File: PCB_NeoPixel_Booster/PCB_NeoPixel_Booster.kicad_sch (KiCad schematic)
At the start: 22 parts, among them J1 Power_Input_Screw, J10 Power_Breakout, J11 Power_Input_Screw, J12 REG_CONTROL, J2 Power_Input_Barrel_Jack, J3 Vcc_Breakout, J4 LED_Strip_Connector, J5 Power_Input_Screw, J6 LED_Strip_Connector, J7 Data_Input, J8 Power_Breakout, U1 AP2210K-5.0, U3 74LVC2G34GW

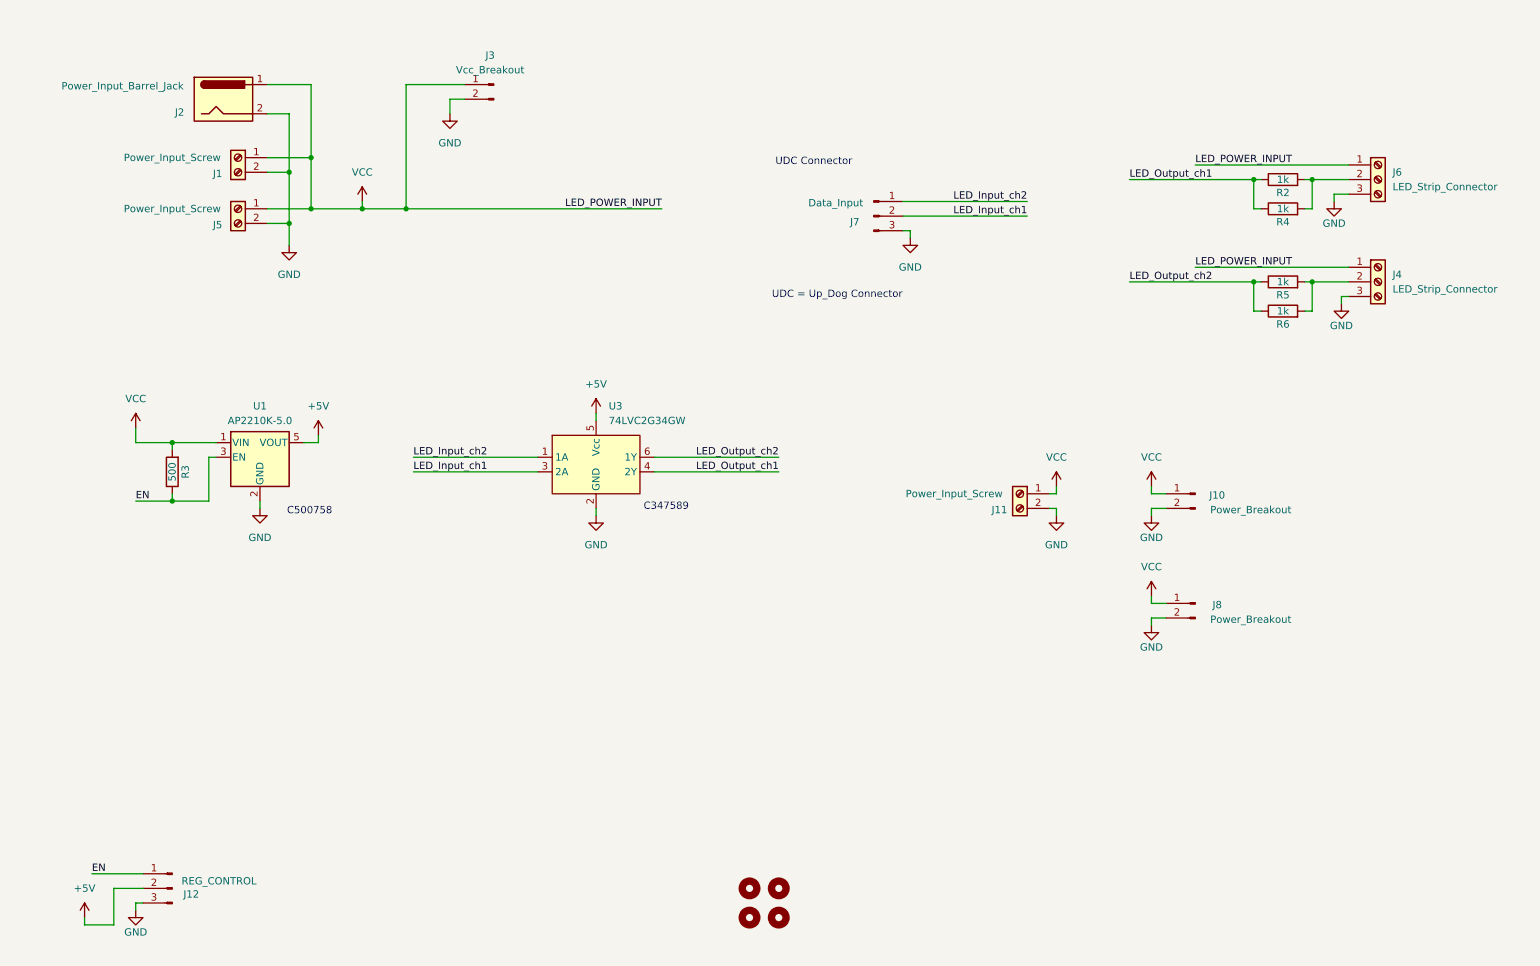
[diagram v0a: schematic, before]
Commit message: Fin
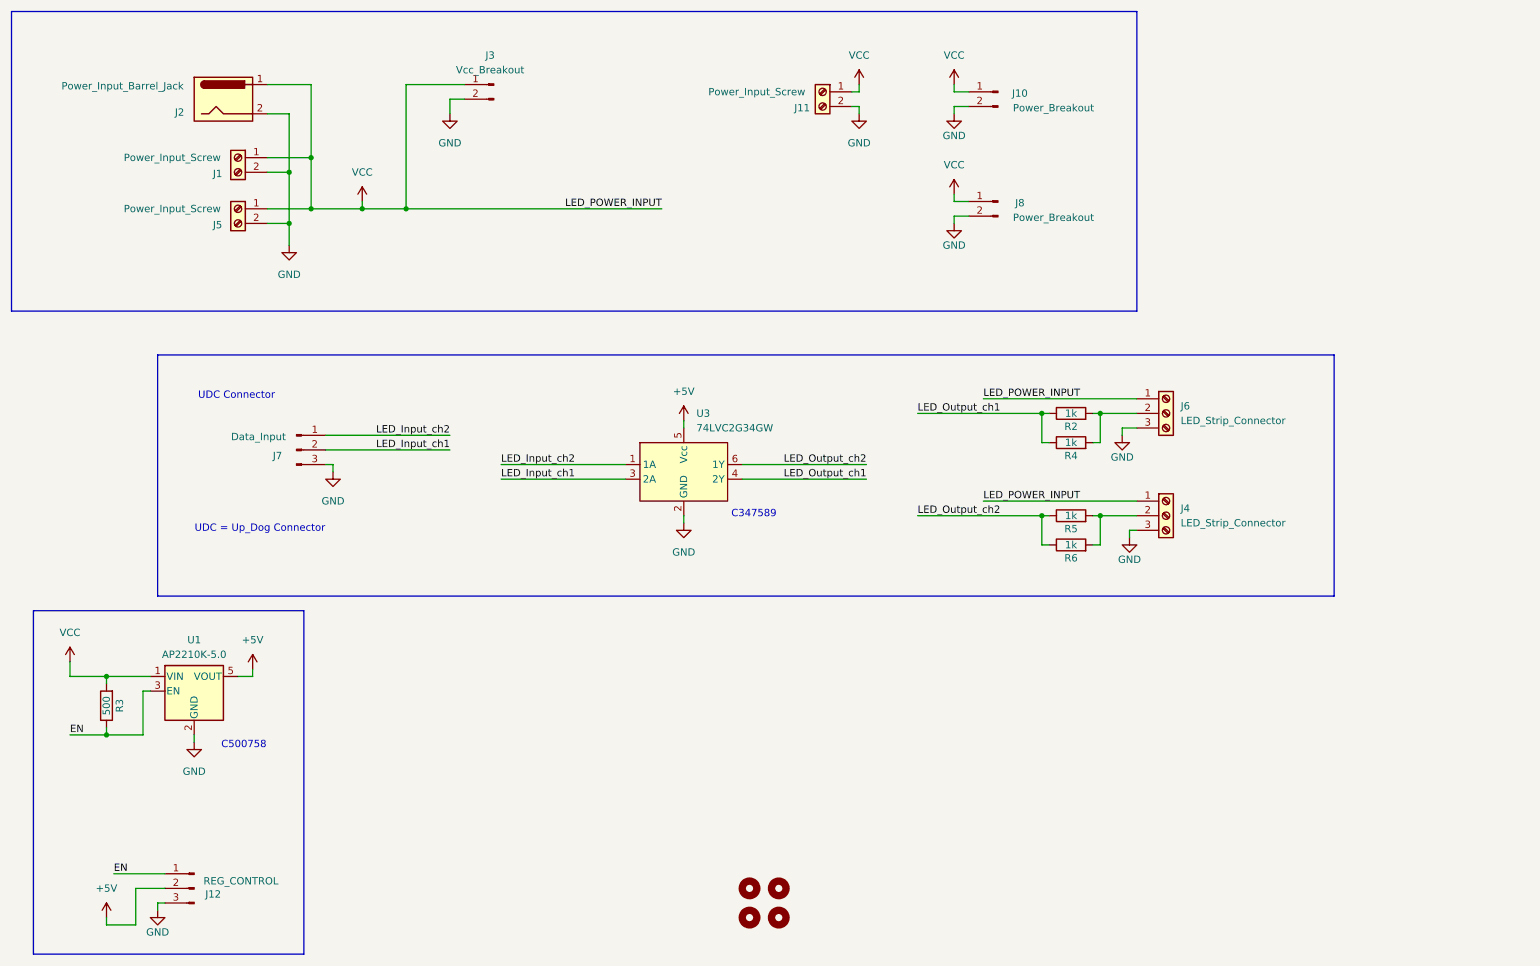
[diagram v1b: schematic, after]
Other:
- moved on the sheet: J10, J11, J12, J4, J6, J7, J8, R2, R3, R4, R5, R6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
